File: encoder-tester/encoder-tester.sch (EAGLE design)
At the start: 6 parts

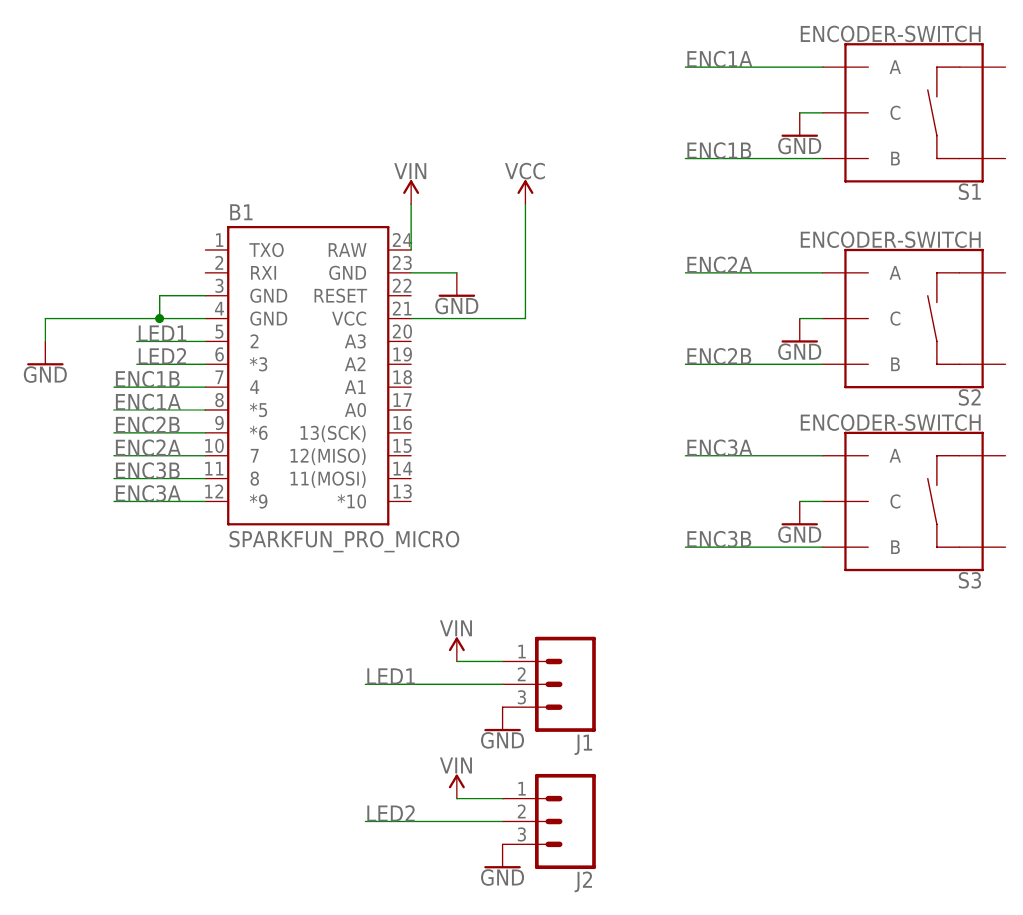
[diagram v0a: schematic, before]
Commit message: board fixups
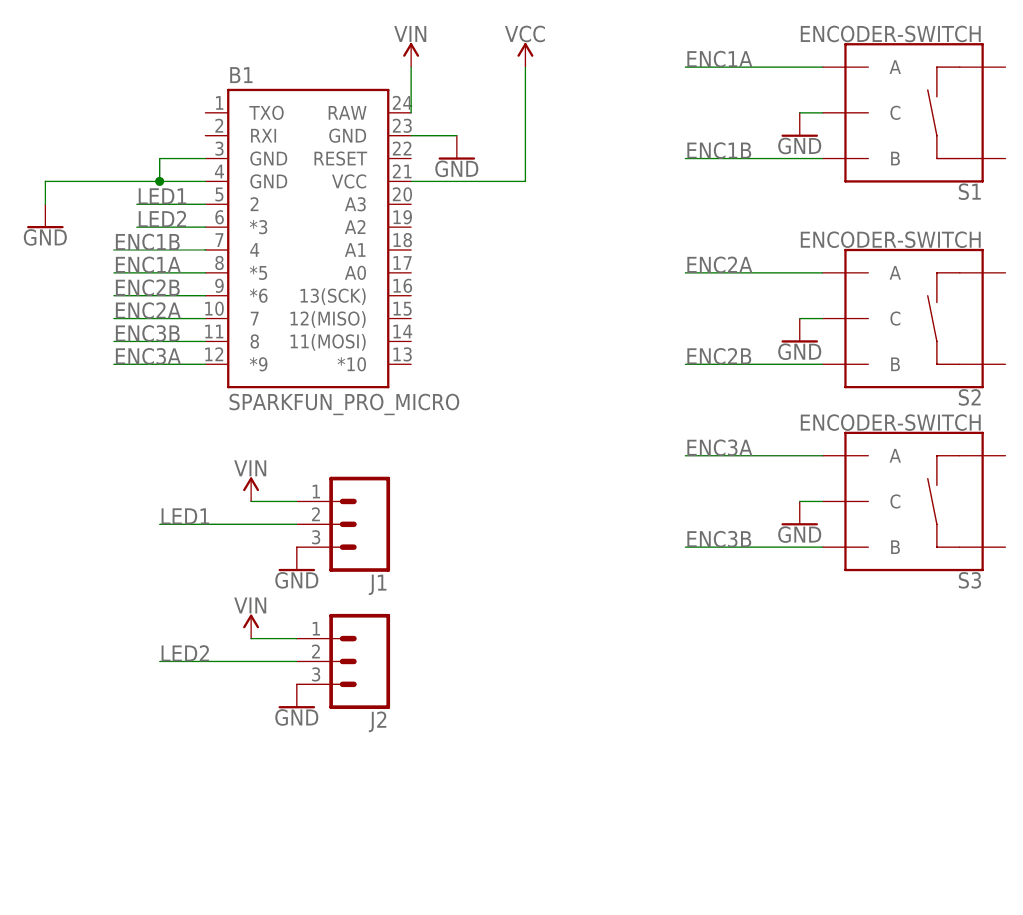
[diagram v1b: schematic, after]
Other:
- moved on the sheet: B1, J1, J2
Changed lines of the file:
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@@
 </plain>
 <instances>
-<instance part="B1" gate="G$1" x="22.86" y="53.34"/>
+<instance part="B1" gate="G$1" x="22.86" y="68.58"/>
 <instance part="S1" gate="G$1" x="91.44" y="83.82" rot="R180"/>
 <instance part="S2" gate="G$1" x="91.44" y="60.96" rot="R180"/>
@@
 <instance part="GND2" gate="1" x="78.74" y="58.42"/>
 <instance part="GND3" gate="1" x="78.74" y="38.1"/>
-<instance part="GND4" gate="1" x="-5.08" y="55.88"/>
-<instance part="SUPPLY1" gate="G$1" x="48.26" y="73.66"/>
-<instance part="GND5" gate="1" x="40.64" y="63.5"/>
-<instance part="SUPPLY2" gate="G$1" x="35.56" y="73.66"/>
-<instance part="J1" gate="J$1" x="53.34" y="20.32" rot="R180"/>
-<instance part="J2" gate="J$1" x="53.34" y="5.08" rot="R180"/>
-<instance part="GND6" gate="1" x="45.72" y="15.24"/>
-<instance part="GND7" gate="1" x="45.72" y="0"/>
-<instance part="SUPPLY3" gate="G$1" x="40.64" y="22.86"/>
-<instance part="SUPPLY4" gate="G$1" x="40.64" y="7.62"/>
+<instance part="GND4" gate="1" x="-5.08" y="71.12"/>
+<instance part="SUPPLY1" gate="G$1" x="48.26" y="88.9"/>
+<instance part="GND5" gate="1" x="40.64" y="78.74"/>
+<instance part="SUPPLY2" gate="G$1" x="35.56" y="88.9"/>
+<instance part="J1" gate="J$1" x="30.48" y="38.1" rot="R180"/>
+<instance part="J2" gate="J$1" x="30.48" y="22.86" rot="R180"/>
+<instance part="GND6" gate="1" x="22.86" y="33.02"/>
+<instance part="GND7" gate="1" x="22.86" y="17.78"/>
+<instance part="SUPPLY3" gate="G$1" x="17.78" y="40.64"/>
+<instance part="SUPPLY4" gate="G$1" x="17.78" y="25.4"/>
 </instances>
 <busses>
@@
 <pinref part="B1" gate="G$1" pin="GND"/>
 <pinref part="GND4" gate="1" pin="GND"/>
-<wire x1="12.7" y1="60.96" x2="7.62" y2="60.96" width="0.1524" layer="91"/>
-<wire x1="7.62" y1="60.96" x2="-5.08" y2="60.96" width="0.1524" layer="91"/>
-<wire x1="-5.08" y1="60.96" x2="-5.08" y2="58.42" width="0.1524" layer="91"/>
+<wire x1="12.7" y1="76.2" x2="7.62" y2="76.2" width="0.1524" layer="91"/>
+<wire x1="7.62" y1="76.2" x2="-5.08" y2="76.2" width="0.1524" layer="91"/>
+<wire x1="-5.08" y1="76.2" x2="-5.08" y2="73.66" width="0.1524" layer="91"/>
 <pinref part="B1" gate="G$1" pin="GND@1"/>
-<wire x1="12.7" y1="63.5" x2="7.62" y2="63.5" width="0.1524" layer="91"/>
-<wire x1="7.62" y1="63.5" x2="7.62" y2="60.96" width="0.1524" layer="91"/>
-<junction x="7.62" y="60.96"/>
+<wire x1="12.7" y1="78.74" x2="7.62" y2="78.74" width="0.1524" layer="91"/>
+<wire x1="7.62" y1="78.74" x2="7.62" y2="76.2" width="0.1524" layer="91"/>
+<junction x="7.62" y="76.2"/>
 </segment>
 <segment>
 <pinref part="B1" gate="G$1" pin="GND@2"/>
 <pinref part="GND5" gate="1" pin="GND"/>
-<wire x1="35.56" y1="66.04" x2="40.64" y2="66.04" width="0.1524" layer="91"/>
+<wire x1="35.56" y1="81.28" x2="40.64" y2="81.28" width="0.1524" layer="91"/>
 </segment>
 <segment>
@@
 <segment>
 <pinref part="B1" gate="G$1" pin="*5"/>
-<wire x1="12.7" y1="50.8" x2="2.54" y2="50.8" width="0.1524" layer="91"/>
-<label x="2.54" y="50.8" size="1.778" layer="95"/>
+<wire x1="12.7" y1="66.04" x2="2.54" y2="66.04" width="0.1524" layer="91"/>
+<label x="2.54" y="66.04" size="1.778" layer="95"/>
 </segment>
 </net>
@@
 <segment>
 <pinref part="B1" gate="G$1" pin="4"/>
-<wire x1="12.7" y1="53.34" x2="2.54" y2="53.34" width="0.1524" layer="91"/>
-<label x="2.54" y="53.34" size="1.778" layer="95"/>
+<wire x1="12.7" y1="68.58" x2="2.54" y2="68.58" width="0.1524" layer="91"/>
+<label x="2.54" y="68.58" size="1.778" layer="95"/>
 </segment>
 </net>
@@
 <segment>
 <pinref part="B1" gate="G$1" pin="7"/>
-<wire x1="12.7" y1="45.72" x2="2.54" y2="45.72" width="0.1524" layer="91"/>
-<label x="2.54" y="45.72" size="1.778" layer="95"/>
+<wire x1="12.7" y1="60.96" x2="2.54" y2="60.96" width="0.1524" layer="91"/>
+<label x="2.54" y="60.96" size="1.778" layer="95"/>
 </segment>
 </net>
@@
 <segment>
 <pinref part="B1" gate="G$1" pin="*6"/>
-<wire x1="12.7" y1="48.26" x2="2.54" y2="48.26" width="0.1524" layer="91"/>
-<label x="2.54" y="48.26" size="1.778" layer="95"/>
+<wire x1="12.7" y1="63.5" x2="2.54" y2="63.5" width="0.1524" layer="91"/>
+<label x="2.54" y="63.5" size="1.778" layer="95"/>
 </segment>
 </net>
@@
 <segment>
 <pinref part="B1" gate="G$1" pin="*9"/>
-<wire x1="12.7" y1="40.64" x2="2.54" y2="40.64" width="0.1524" layer="91"/>
-<label x="2.54" y="40.64" size="1.778" layer="95"/>
+<wire x1="12.7" y1="55.88" x2="2.54" y2="55.88" width="0.1524" layer="91"/>
+<label x="2.54" y="55.88" size="1.778" layer="95"/>
 </segment>
 </net>
@@
 <segment>
 <pinref part="B1" gate="G$1" pin="8"/>
-<wire x1="12.7" y1="43.18" x2="2.54" y2="43.18" width="0.1524" layer="91"/>
-<label x="2.54" y="43.18" size="1.778" layer="95"/>
+<wire x1="12.7" y1="58.42" x2="2.54" y2="58.42" width="0.1524" layer="91"/>
+<label x="2.54" y="58.42" size="1.778" layer="95"/>
 </segment>
 </net>
@@
 <segment>
 <pinref part="B1" gate="G$1" pin="VCC"/>
-<wire x1="35.56" y1="60.96" x2="48.26" y2="60.96" width="0.1524" layer="91"/>
-<wire x1="48.26" y1="60.96" x2="48.26" y2="73.66" width="0.1524" layer="91"/>
+<wire x1="35.56" y1="76.2" x2="48.26" y2="76.2" width="0.1524" layer="91"/>
+<wire x1="48.26" y1="76.2" x2="48.26" y2="88.9" width="0.1524" layer="91"/>
 <pinref part="SUPPLY1" gate="G$1" pin="VCC"/>
 </segment>
@@
 <pinref part="B1" gate="G$1" pin="RAW"/>
 <pinref part="SUPPLY2" gate="G$1" pin="VIN"/>
-<wire x1="35.56" y1="68.58" x2="35.56" y2="73.66" width="0.1524" layer="91"/>
+<wire x1="35.56" y1="83.82" x2="35.56" y2="88.9" width="0.1524" layer="91"/>
 </segment>
 <segment>
 <pinref part="J1" gate="J$1" pin="1"/>
 <pinref part="SUPPLY3" gate="G$1" pin="VIN"/>
-<wire x1="40.64" y1="22.86" x2="45.72" y2="22.86" width="0.1524" layer="91"/>
+<wire x1="17.78" y1="40.64" x2="22.86" y2="40.64" width="0.1524" layer="91"/>
 </segment>
 <segment>
 <pinref part="J2" gate="J$1" pin="1"/>
 <pinref part="SUPPLY4" gate="G$1" pin="VIN"/>
-<wire x1="40.64" y1="7.62" x2="45.72" y2="7.62" width="0.1524" layer="91"/>
+<wire x1="17.78" y1="25.4" x2="22.86" y2="25.4" width="0.1524" layer="91"/>
 </segment>
 </net>
@@
 <segment>
 <pinref part="B1" gate="G$1" pin="2"/>
-<wire x1="12.7" y1="58.42" x2="5.08" y2="58.42" width="0.1524" layer="91"/>
-<label x="5.08" y="58.42" size="1.778" layer="95"/>
+<wire x1="12.7" y1="73.66" x2="5.08" y2="73.66" width="0.1524" layer="91"/>
+<label x="5.08" y="73.66" size="1.778" layer="95"/>
 </segment>
 <segment>
 <pinref part="J1" gate="J$1" pin="2"/>
-<wire x1="45.72" y1="20.32" x2="30.48" y2="20.32" width="0.1524" layer="91"/>
-<label x="30.48" y="20.32" size="1.778" layer="95"/>
+<wire x1="22.86" y1="38.1" x2="7.62" y2="38.1" width="0.1524" layer="91"/>
+<label x="7.62" y="38.1" size="1.778" layer="95"/>
 </segment>
 </net>
@@
 <segment>
 <pinref part="B1" gate="G$1" pin="*3"/>
-<wire x1="12.7" y1="55.88" x2="5.08" y2="55.88" width="0.1524" layer="91"/>
-<label x="5.08" y="55.88" size="1.778" layer="95"/>
+<wire x1="12.7" y1="71.12" x2="5.08" y2="71.12" width="0.1524" layer="91"/>
+<label x="5.08" y="71.12" size="1.778" layer="95"/>
 </segment>
 <segment>
 <pinref part="J2" gate="J$1" pin="2"/>
-<wire x1="45.72" y1="5.08" x2="30.48" y2="5.08" width="0.1524" layer="91"/>
-<label x="30.48" y="5.08" size="1.778" layer="95"/>
+<wire x1="22.86" y1="22.86" x2="7.62" y2="22.86" width="0.1524" layer="91"/>
+<label x="7.62" y="22.86" size="1.778" layer="95"/>
 </segment>
 </net>
